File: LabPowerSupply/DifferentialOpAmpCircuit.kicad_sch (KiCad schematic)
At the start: 12 parts

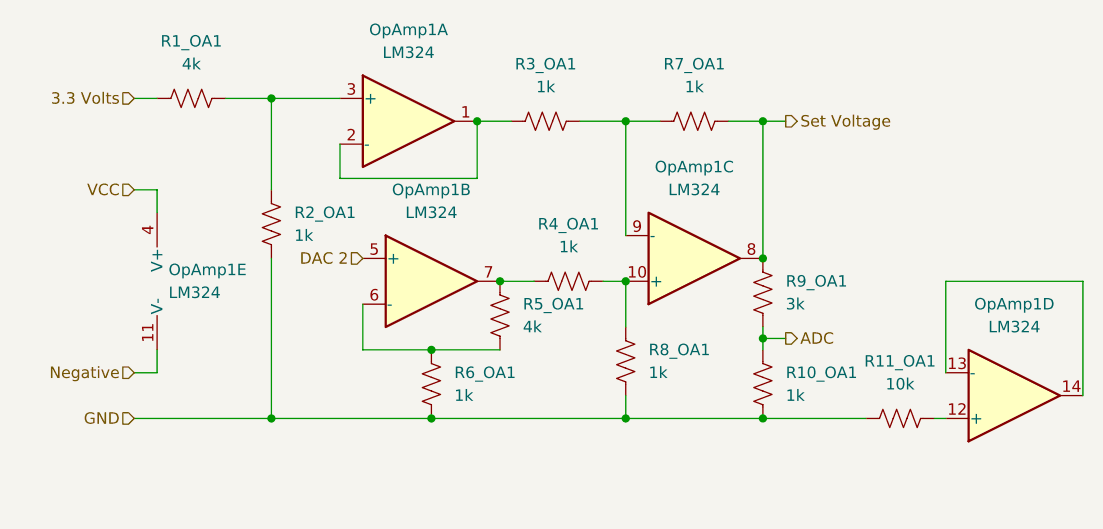
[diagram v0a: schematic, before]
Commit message: almost done
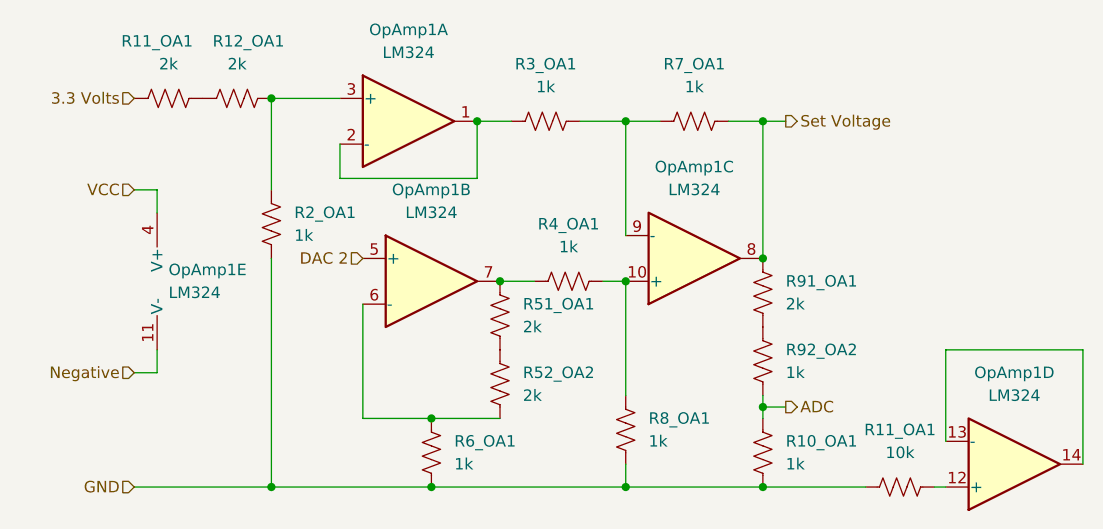
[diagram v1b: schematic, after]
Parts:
- removed R1_OA1: 4k, Resistor_SMD:R_0603_1608Metric, symbol Device:R_US
- added R11_OA1, R12_OA1: 2k, symbol Device:R_US
- added R52_OA2: 2k, Resistor_SMD:R_0603_1608Metric, symbol Device:R_US
- added R92_OA2: 1k, Resistor_SMD:R_0603_1608Metric, symbol Device:R_US
- R51_OA1: renamed from R5_OA1; value 4k -> 2k
- R91_OA1: renamed from R9_OA1; value 3k -> 2k
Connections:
- net 3.3 Volts: now also R11_OA1.1
- net ADC: now also R92_OA2.2; no longer R91_OA1.2
- net at OpAmp1.3 (+), R2_OA1.1: now also R12_OA1.2
- net at OpAmp1.6 (-), R6_OA1.1: now also R52_OA2.2; no longer R51_OA1.2
- new net: R91_OA1.2, R92_OA2.1
- new net: R51_OA1.2, R52_OA2.1
- new net: R11_OA1.2, R12_OA1.1
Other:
- moved on the sheet: OpAmp1D, R10_OA1, R11_OA1, R6_OA1, R8_OA1
